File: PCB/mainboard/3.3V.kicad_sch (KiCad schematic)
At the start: 12 parts, among them U2 TPS5430DDA

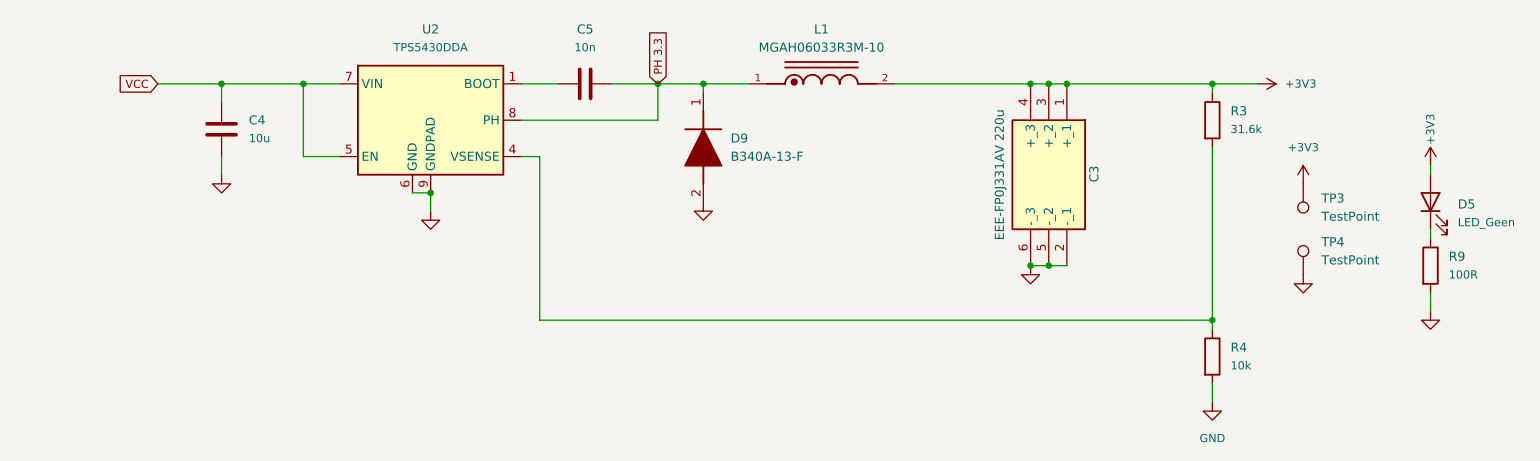
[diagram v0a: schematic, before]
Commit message: random upload
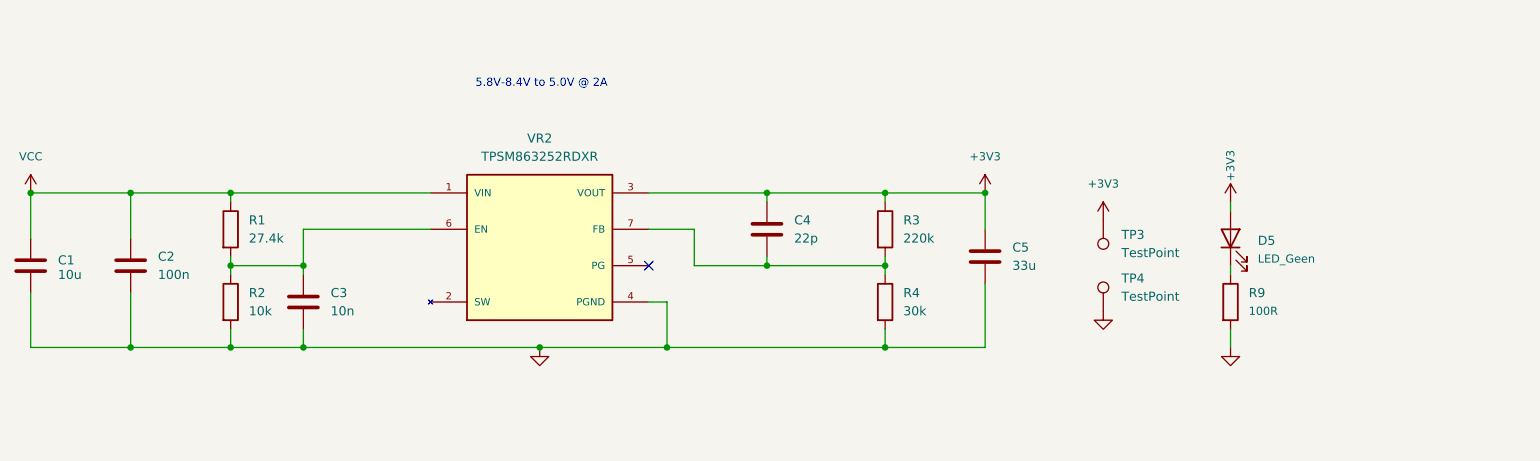
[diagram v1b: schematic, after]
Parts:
- removed C3: EEE-FP0J331AV 220u, lib:EEEFP0J331AV, symbol EEE-FP0J331AV:EEE-FP0J331AV
- removed D9: B340A-13-F, lib:DIOM5226X240N, symbol B340A-13-F:B340A-13-F
- removed L1: MGAH06033R3M-10, lib:IND_MGAH06033R3M-10, symbol MGAH06033R3M-10:MGAH06033R3M-10
- removed U2: TPS5430DDA, Package_SO:TI_SO-PowerPAD-8_ThermalVias, symbol Regulator_Switching:TPS5430DDA
- added C1: 10u, Capacitor_SMD:C_0402_1005Metric_Pad0.74x0.62mm_HandSolder, symbol Device:C
- added C2: 100n, Capacitor_SMD:C_0402_1005Metric_Pad0.74x0.62mm_HandSolder, symbol Device:C
- added C3: 10n, Capacitor_SMD:C_0402_1005Metric_Pad0.74x0.62mm_HandSolder, symbol Device:C
- added R1: 27.4k, Resistor_SMD:R_0402_1005Metric_Pad0.72x0.64mm_HandSolder, symbol Device:R
- added R2: 10k, Resistor_SMD:R_0402_1005Metric_Pad0.72x0.64mm_HandSolder, symbol Device:R
- added VR2: TPSM863252RDXR, lib:VREG_TPSM863252RDXR, symbol TPSM863252RDXR:TPSM863252RDXR
- C4: value 10u -> 22p; footprint Capacitor_SMD:C_1206_3216Metric_Pad1.33x1.80mm_HandSolder -> Capacitor_SMD:C_0402_1005Metric_Pad0.74x0.62mm_HandSolder
- C5: value 10n -> 33u; footprint Capacitor_SMD:C_1206_3216Metric_Pad1.33x1.80mm_HandSolder -> lib:C4532_Commercial
- R3: value 31.6k -> 220k
- R4: value 10k -> 30k
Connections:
- net PH 3.3 is gone; now on net GND: C5.2
- net +3V3: now also C4.1, C5.1, VR2.3 (VOUT)
- net GND: now also C1.2, C2.2, C3.2, R2.2, VR2.4 (PGND); no longer C4.2
- net VCC: now also C1.1, C2.1, R1.1, VR2.1 (VIN); no longer C4.1
- net at R3.2, R4.1: now also C4.2, VR2.7 (FB)
- new net: C3.1, R1.2, R2.1, VR2.6 (EN)
- no-connect marks 0 -> 1
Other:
- note added: "5.8V-8.4V to 5.0V @ 2A"
- moved on the sheet: D5, R9, TP3, TP4
